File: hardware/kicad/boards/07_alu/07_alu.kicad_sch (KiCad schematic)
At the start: 19 parts, among them J1 Conn_01x08_Pin, J10 Conn_01x04_Pin, J11 Conn_01x04_Pin, J2 Conn_01x08_Pin, J3 Conn_01x08_Pin, J4 Conn_01x08_Pin, J5 Conn_01x08_Pin, J6 Conn_01x08_Pin, J7 Conn_01x08_Pin, J8 Conn_01x08_Pin, J9 Conn_01x08_Pin, U1 74ACT151, U2 74ACT151, U35 74AHC1G04

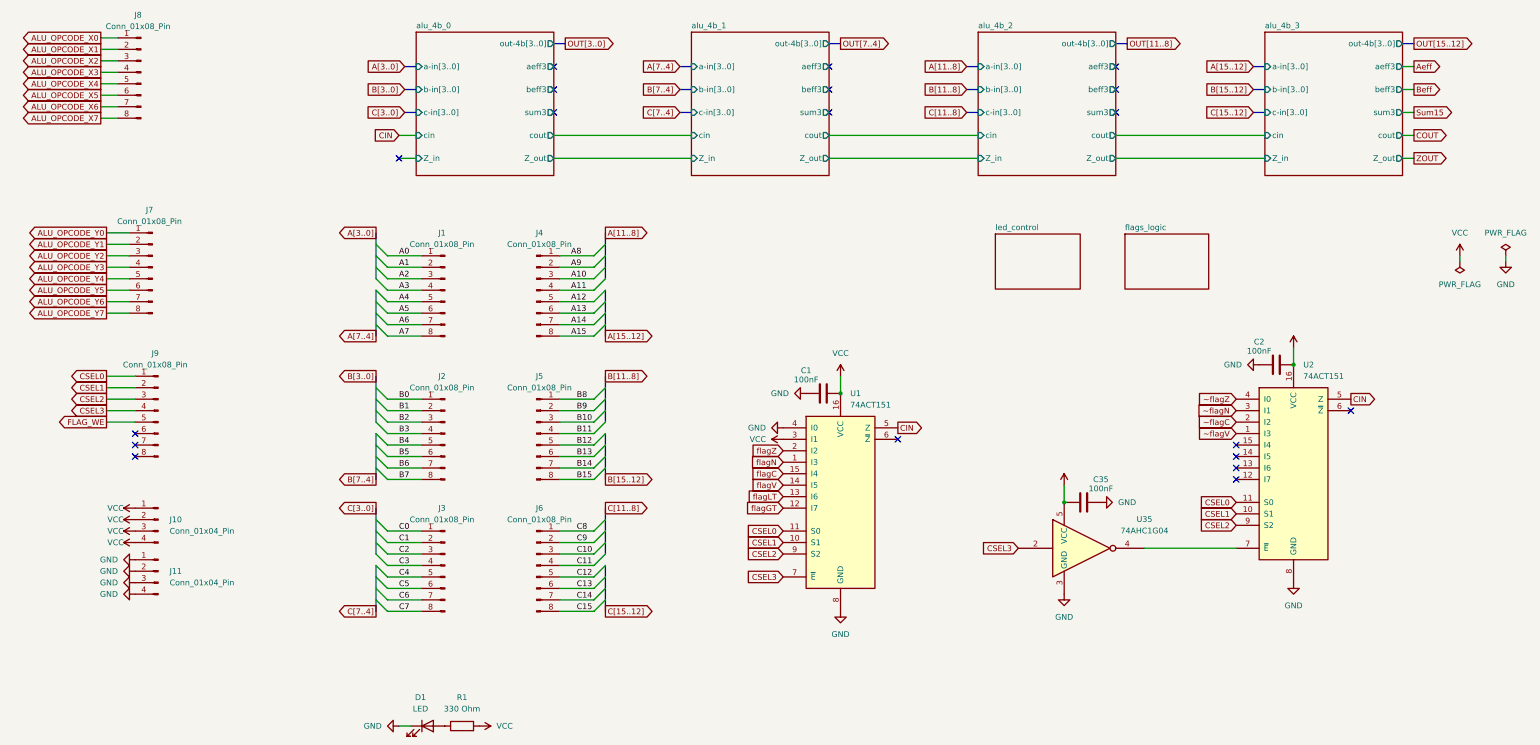
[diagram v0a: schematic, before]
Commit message: checkpoint: most recent 16b cell: ~120mm by 120mm
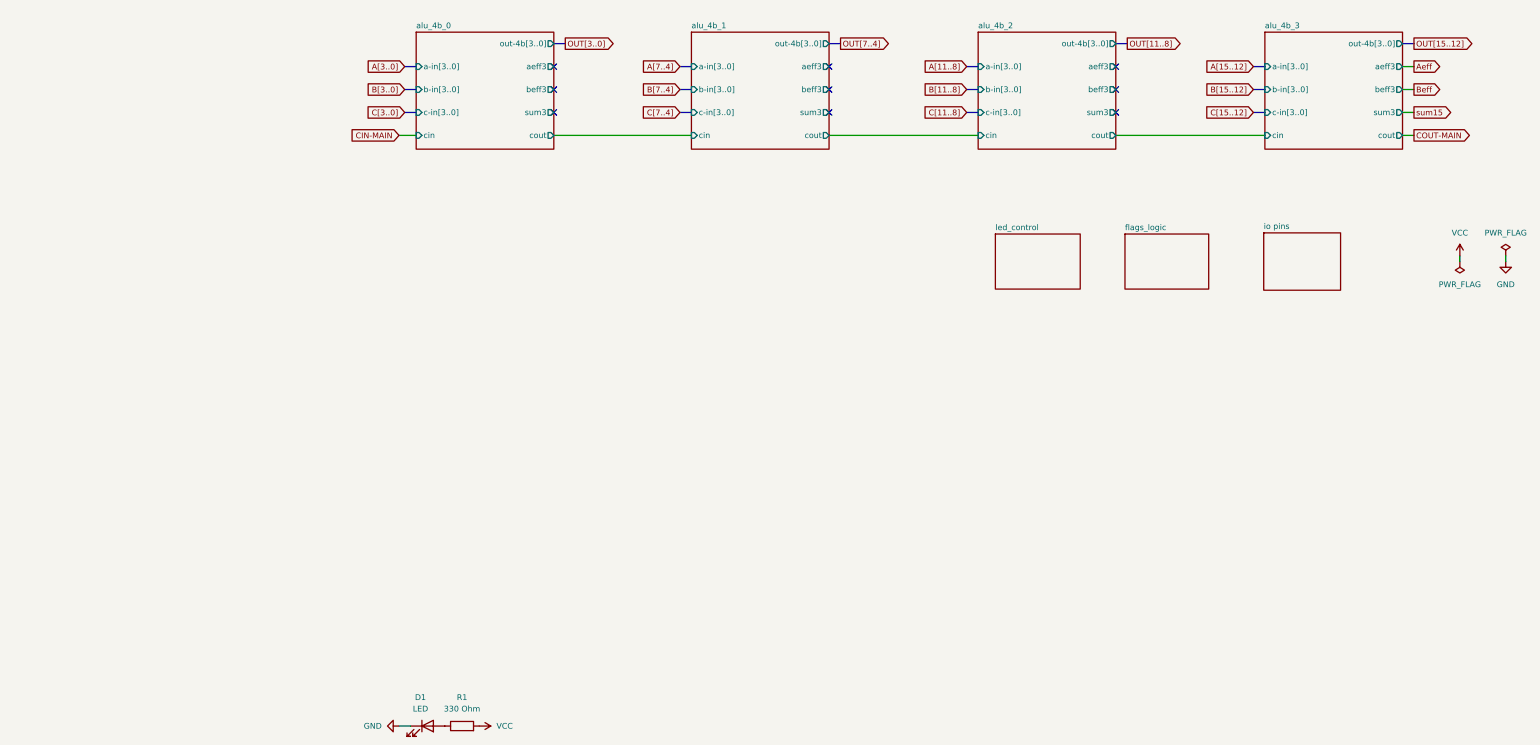
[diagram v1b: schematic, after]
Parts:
- removed C1, C2, C35: 100nF, Capacitor_SMD:C_0603_1608Metric, symbol Device:C
- removed J1, J2, J3, J4, J5, J6, J7, J8, J9: Conn_01x08_Pin, Connector_PinHeader_2.54mm:PinHeader_1x08_P2.54mm_Vertical, symbol Connector:Conn_01x08_Pin
- removed J10, J11: Conn_01x04_Pin, Connector_PinHeader_2.54mm:PinHeader_1x04_P2.54mm_Vertical, symbol Connector:Conn_01x04_Pin
- removed U1, U2: 74ACT151, Package_SO:SOIC-16_3.9x9.9mm_P1.27mm, symbol 74xx:74LS151
- removed U35: 74AHC1G04, Package_TO_SOT_SMD:SOT-23-5, symbol 74xGxx:74AHC1G04
- D1: footprint LED_THT:LED_D5.0mm -> LED_SMD:LED_0805_2012Metric
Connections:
- no-connect marks 19 -> 9
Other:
- added sheet io pins (iopins.kicad_sch)
- sheet alu_4b_0 ports: added none; removed Z_in, Z_out
- sheet alu_4b_1 ports: added none; removed Z_in, Z_out
- sheet alu_4b_2 ports: added none; removed Z_in, Z_out
- sheet alu_4b_3 ports: added none; removed Z_in, Z_out
